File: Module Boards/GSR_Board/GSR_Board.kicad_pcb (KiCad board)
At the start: 4 copper layers, 23.4 x 10.7 mm, 71 parts, among them U1 AD8236ARMZ-R7, U2 LTC2064IDD#PBF, U3 MAX5419LETA+T, U4 MAX5419LETA+T, U5 TPS7A9401DSCR, U6 TXS0102DQER, U7 LTC1864LIMS8#PBF, U8 TXB0104RUTR, U9 TPS22916CYFPR

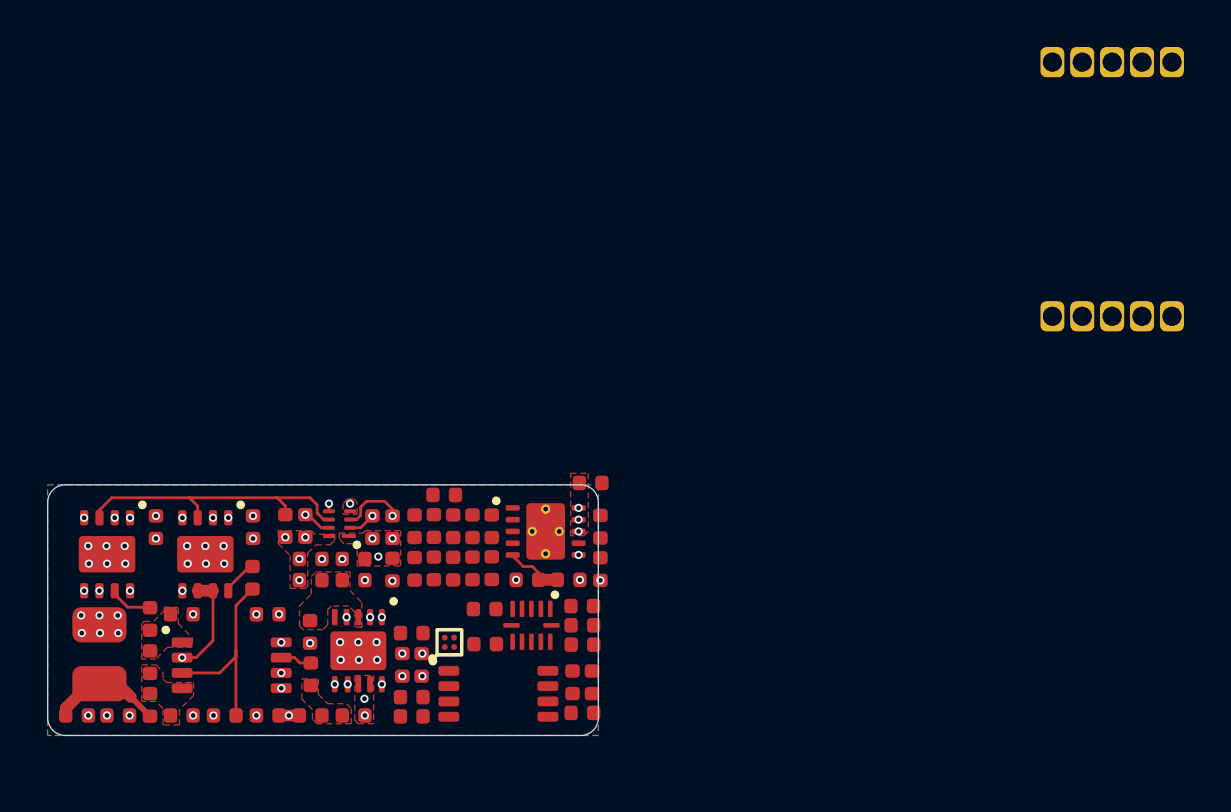
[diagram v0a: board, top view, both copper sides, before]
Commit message: Finished Routing of GSR Board
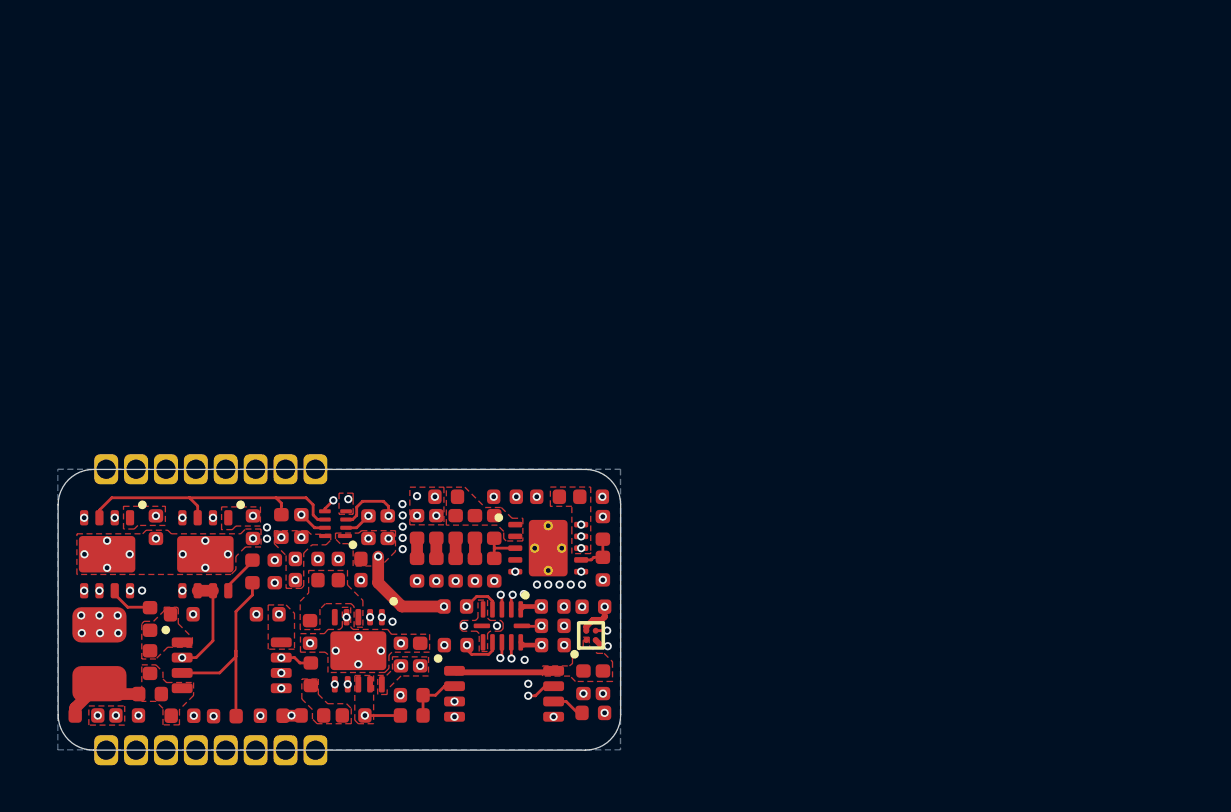
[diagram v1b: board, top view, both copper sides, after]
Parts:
- U5: footprint X-MODs_PcbLib:WSON-8-3.15x3.15mm -> X-MODs_PcbLib:WSON-10-3.15x3.15mm
- moved J2 30.8 mm to (127.9, 94.0)
- moved C25 7.80 mm to (138.9, 94.0)
- moved U9 6.02 mm to (138.8, 95.2)
- moved R5 5.00 mm to (125.4, 92.5)
- moved R18 4.45 mm to (138.8, 89.3)
- moved R19 4.44 mm to (135.2, 89.3), turned to 180 degrees
- moved C17 1.90 mm to (137.0, 89.3), turned to 180 degrees
- moved C23 1.26 mm to (137.2, 94.0)
- moved C24 1.26 mm to (137.2, 95.6)
- moved R20 1.26 mm to (137.2, 94.8)
- moved R29 1.26 mm to (133.1, 95.6)
- moved U8 1.26 mm to (135.1, 94.8)
- moved R28 1.25 mm to (133.1, 94.0)
- moved U5 0.72 mm to (137.0, 91.5)
- moved C22 0.46 mm to (139.3, 97.2)
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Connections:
- J2 pad 1: GSR -> GND
- J2 pad 10: SCL_1V8 -> +1V8
- J2 pad 2: GND -> LVL_SHIFTER_EN
- J2 pad 3: +1V8 -> GND
- J2 pad 4: GND -> ADC_EN
- J2 pad 5: +3V3 -> GND
- J2 pad 6: LVL_SHIFTER_EN -> V_IA_OUT
- J2 pad 8: SDA_1V8 -> GSR
- J2 pad 9: GND -> +3V3
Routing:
- net ADC_EN: track 0.00 -> 24.8 mm, vias 0 -> 2
- net SPI_CS_1V8: track 0.00 -> 21.2 mm, vias 0 -> 1
- net SPI_SCK_1V8: track 0.00 -> 19.7 mm, vias 0 -> 1
- net SPI_MISO_1V8: track 0.00 -> 19.3 mm, vias 0 -> 1
- net +1V8: track 2.19 -> 15.5 mm, vias 3 -> 5
- net LVL_SHIFTER_EN: track 17.0 -> 28.6 mm
- net V_IA_OUT: track 1.35 -> 11.9 mm, vias 0 -> 2
- net SPI_CS_3V: track 0.00 -> 7.48 mm, vias 0 -> 2
- net SPI_MISO_3V: track 0.00 -> 6.99 mm, vias 0 -> 2
- net +3V3: track 0.00 -> 4.79 mm, vias 0 -> 4
- net Net-(U5-FB_PG): track 2.53 -> 7.29 mm, vias 0 -> 3
- net +3VA_ADC: track 0.00 -> 4.26 mm
- net SPI_SCK_3V: track 0.00 -> 4.07 mm, vias 0 -> 2
- net SCL_1V8: track 5.48 -> 8.89 mm
- net +3VA: track 0.00 -> 2.50 mm, vias 22 -> 20
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- added copper zone on In2.Cu, net +1V8
- added copper zone on F.Cu, net +3V3
- added copper zone on In2.Cu, net +3V3
- added copper zone on In3.Cu, net +3VA
- added copper zone on F.Cu, net +3VA_ADC
- added copper zone on F.Cu, net /[1] Power Regulation & Level Shifting/+3V3_FILT
- added copper zone on B.Cu, net GND
- removed copper zone on B.Cu, net +3VA
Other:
- board size 23.4 x 10.7 mm -> 23.9 x 11.9 mm
- copper layers 4 -> 6
